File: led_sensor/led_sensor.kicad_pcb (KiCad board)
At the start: 4 copper layers, 45 parts

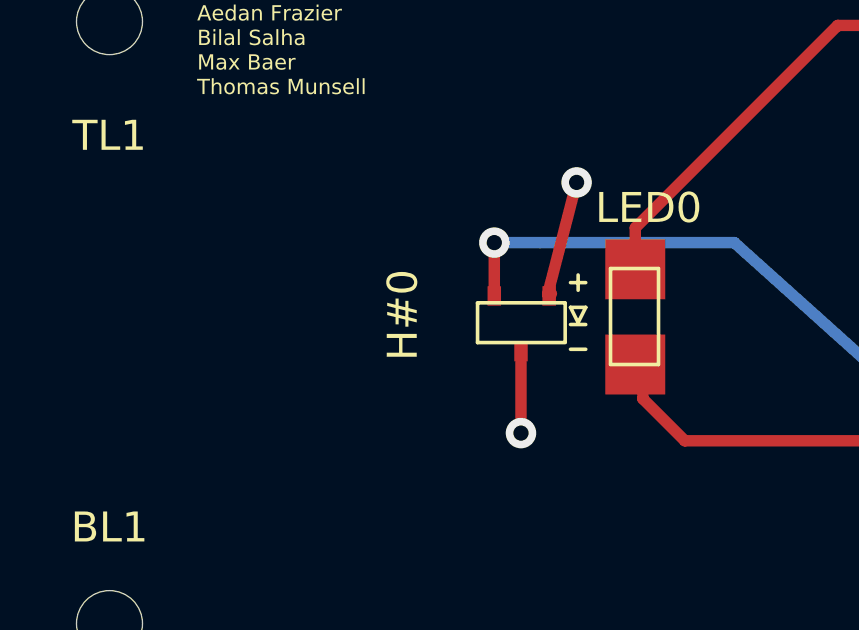
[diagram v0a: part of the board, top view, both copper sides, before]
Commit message: screenshots
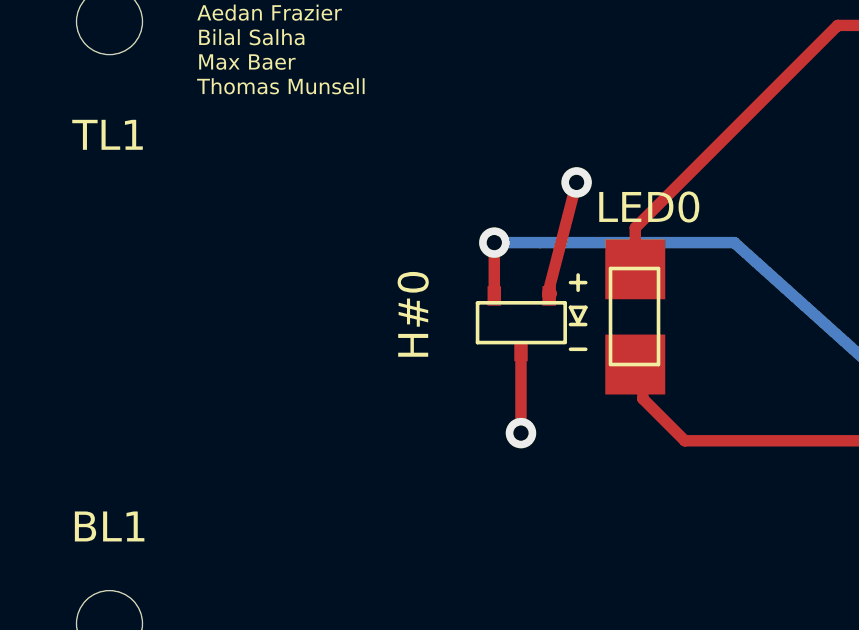
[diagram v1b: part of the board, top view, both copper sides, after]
